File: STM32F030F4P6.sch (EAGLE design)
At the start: 24 parts, among them J3 455-1750-1-ND, J4 CORTEX_DEBUG_MINIMUM_PTH, U1 STM32F030F4P6, U2 CJA1117B-3.3-SOT89

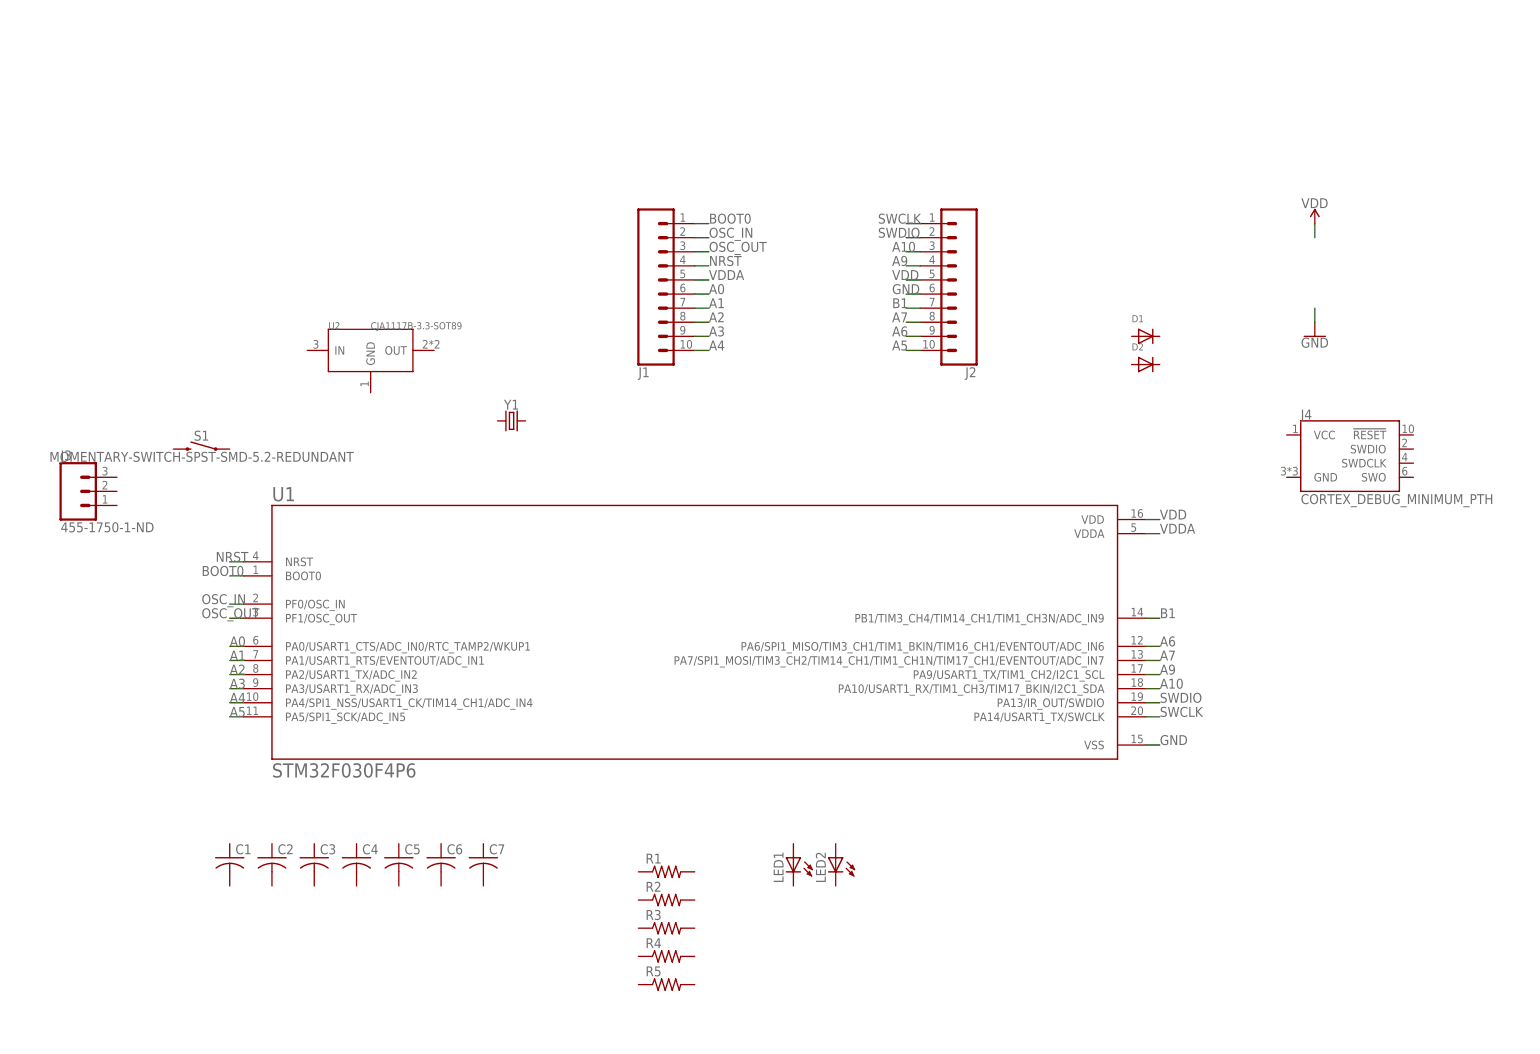
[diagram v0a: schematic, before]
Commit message: Connected all components.
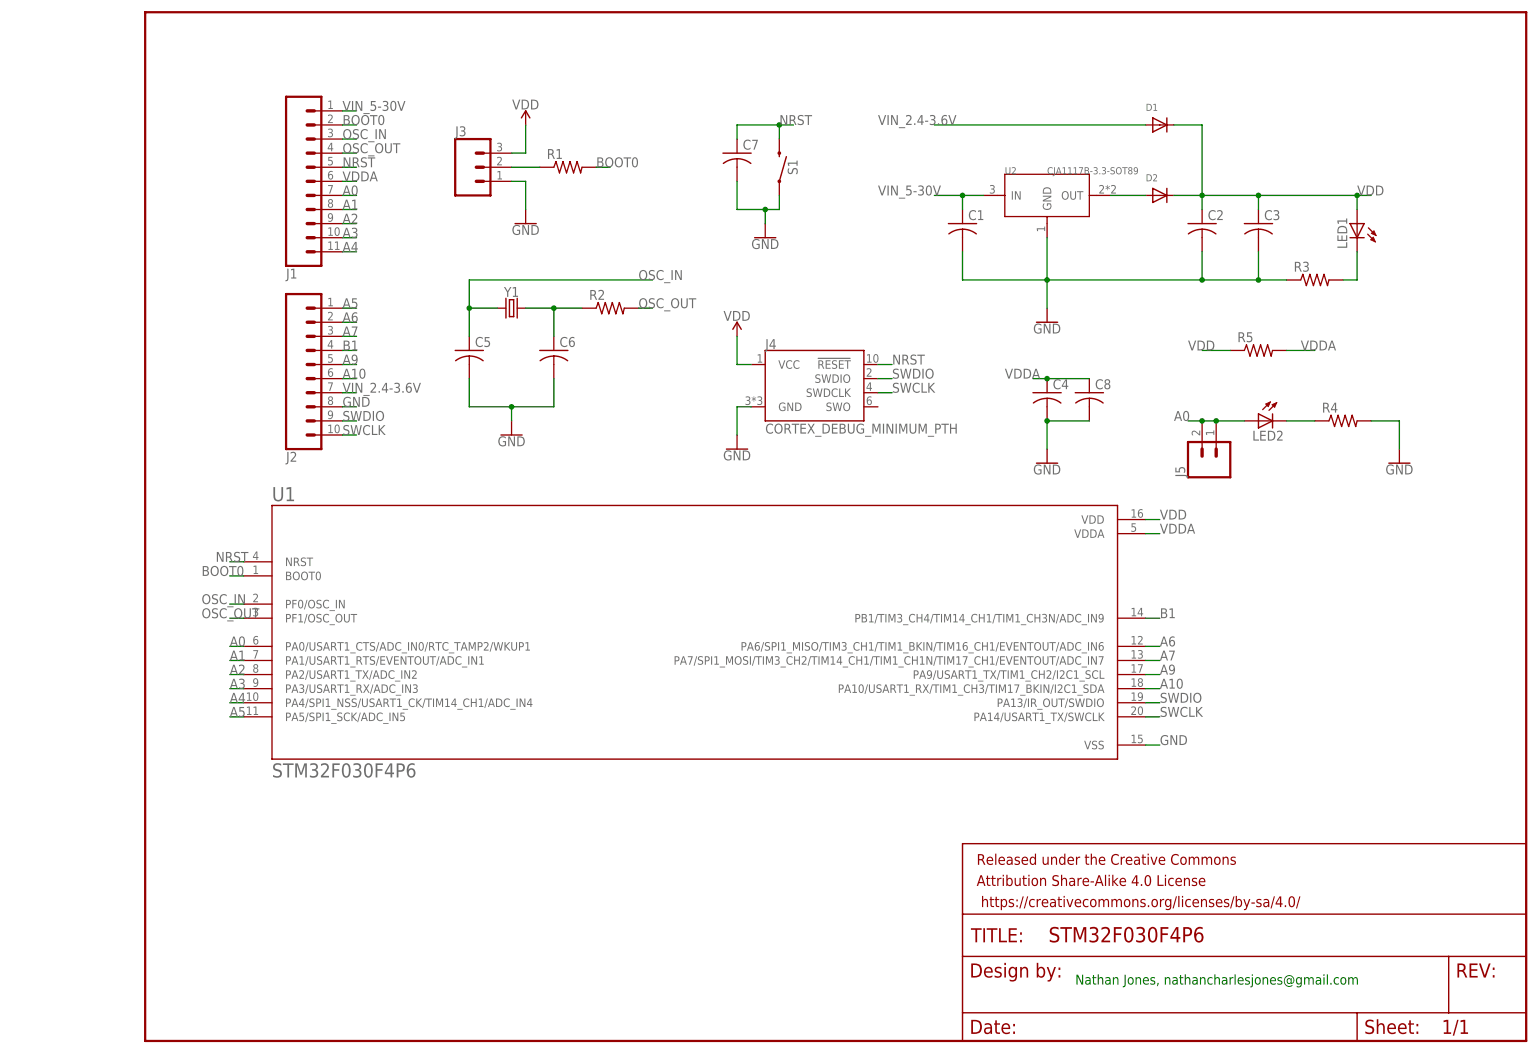
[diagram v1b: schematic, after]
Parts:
- added C8: (no value), adafruit:C-USC0603
- added FRAME1: FRAME-LETTER, SparkFun-Aesthetics:FRAME-LETTER
- added J5: (no value), SparkFun-Connectors:CONN_02
- J1: device SparkFun-Connectors:CONN_10" -> SparkFun-Connectors:CONN_11
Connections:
- new net N$1: J3.2, R1.1
- new net N$3: C6.1, R2.1, Y1.1
- new net N$5: D2.A, U2.OUT
- new net N$7: LED1.C, R3.2
- new net N$8: LED2.C, R4.1
- new net VIN_2.4-3.6V: D1.A, J2.7
- new net VIN_5-30V: C1.1, J1.1, U2.IN
- net A0: now also J1.7, J5.1, J5.2, LED2.A; no longer J1.6
- net A1: now also J1.8; no longer J1.7
- net A10: now also J2.6; no longer J2.3
- net A2: now also J1.9; no longer J1.8
- net A3: now also J1.10; no longer J1.9
- net A4: now also J1.11; no longer J1.10
- net A5: now also J2.1; no longer J2.10
- net A6: now also J2.2; no longer J2.9
- net A7: now also J2.3; no longer J2.8
- net A9: now also J2.5; no longer J2.4
- net B1: now also J2.4; no longer J2.7
- net BOOT0: now also J1.2, R1.2; no longer J1.1
- net GND: now also C1.2, C2.2, C3.2, C4.2, C5.2, C6.2, C7.2, C8.2, J2.8, J3.1, J4.GND, R3.1, R4.2, S1.1, U2.GND; no longer J2.6
- net NRST: now also C7.1, J1.5, J4.!RESET, S1.2; no longer J1.4
- net OSC_IN: now also C5.1, J1.3, Y1.2; no longer J1.2
- net OSC_OUT: now also J1.4, R2.2; no longer J1.3
- net SWCLK: now also J2.10, J4.SWDCLK; no longer J2.1
- net SWDIO: now also J2.9, J4.SWDIO; no longer J2.2
- net VDD: now also C2.1, C3.1, D1.C, D2.C, J3.3, J4.VCC, LED1.A, R5.1; no longer J2.5
- net VDDA: now also C4.1, C8.1, J1.6, R5.2; no longer J1.5
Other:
- note added: "Nathan Jones, nathancharlesjones@gmail.com"
- moved on the sheet: C1, C2, C3, C4, C5, C6, C7, D1, D2, J2, J3, J4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
